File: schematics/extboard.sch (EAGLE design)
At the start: 37 parts, among them X1 FPS009-3000

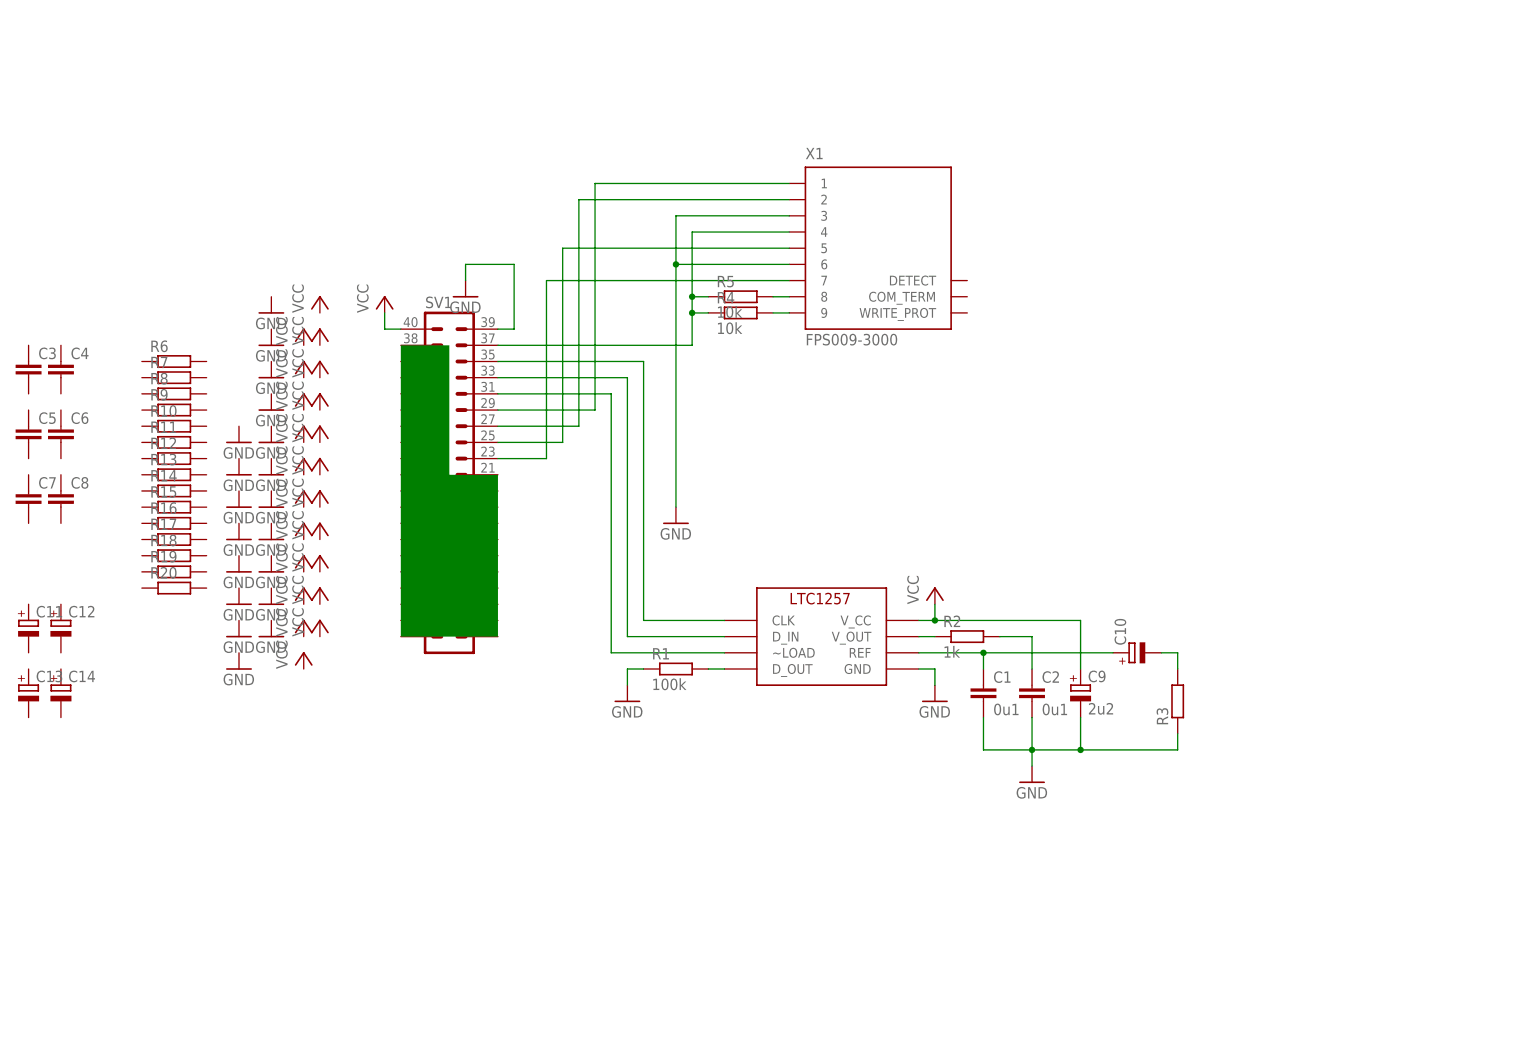
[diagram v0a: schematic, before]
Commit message: schematics: board rev. A
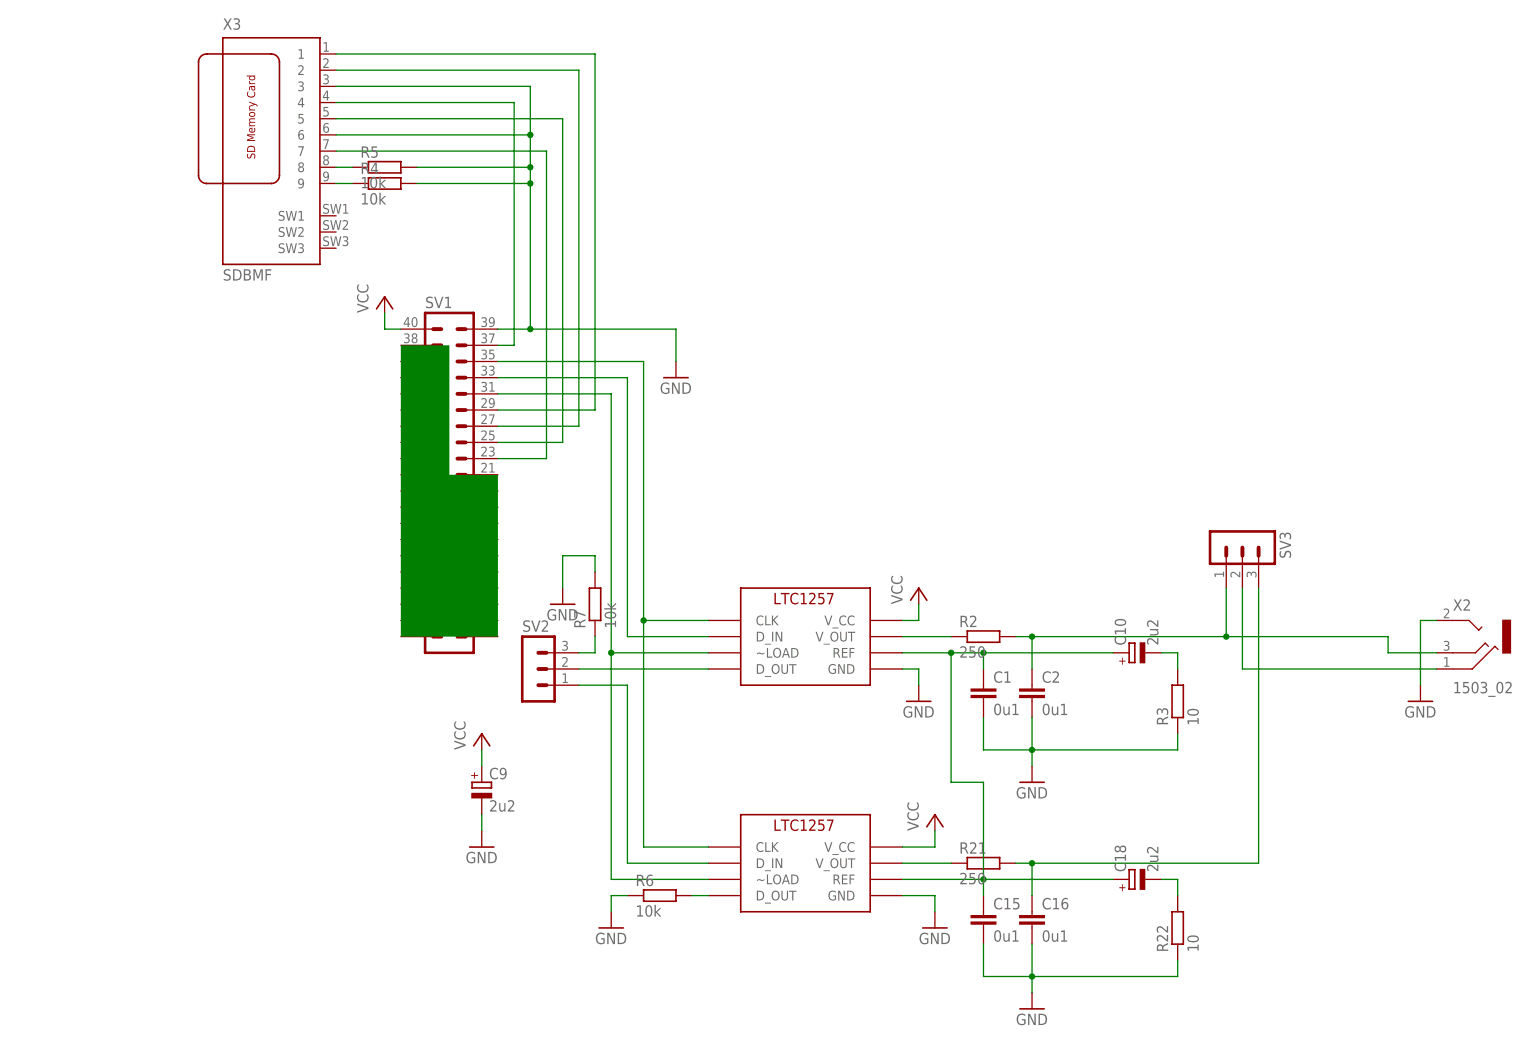
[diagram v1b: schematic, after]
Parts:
- removed C11, C12, C13, C14: (no value), rcl:CPOL-EUE2.5-7
- removed C3, C4, C5, C6, C7, C8: (no value), rcl:C-EU050-035X075
- removed R1: 100k, rcl:R-EU_0207/10
- removed R10, R11, R12, R13, R14, R15, R16, R17, R18, R19, R20, R8, R9: (no value), rcl:R-EU_0207/10
- removed X1: FPS009-3000, con-yamaichi:FPS009-3000
- added C15, C16: 0u1, rcl:C-EU050-035X075
- added C18: 2u2, rcl:CPOL-EUE2.5-7
- added R21: 250, rcl:R-EU_0207/10
- added R22: 10, rcl:R-EU_0207/10
- added SV2, SV3: (no value), con-lstb:MA03-1
- added U$2: LTC1257, ltc1257:LTC1257
- added X2: 1503_02, con-lumberg:1503_02
- added X3: SDBMF, farnell-sd:SDBMF
- C10: value (none) -> 2u2
- R2: value 1k -> 250
- R3: value (none) -> 10
- R6, R7: value (none) -> 10k
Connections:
- new net N$16: R7.1, SV2.3
- new net N$17: SV2.2, U$1.D_OUT
- new net N$18: SV3.2, X2.1
- new net N$19: R6.2, U$2.D_OUT
- new net N$21: C16.1, R21.2, SV3.3
- new net N$22: R21.1, U$2.V_OUT
- new net N$23: C18.-, R22.2
- net GND: now also C15.2, C16.2, R22.1, R4.2, R5.2, R6.1, R7.2, U$2.GND, X2.2, X3.3, X3.6; no longer R1.1, X1.3, X1.6
- net N$1: now also U$2.CLK
- net N$10: now also R4.1, X3.9; no longer R4.2, X1.9
- net N$11: now also X3.4; no longer R4.1, R5.1, X1.4
- net N$12: now also X3.1; no longer X1.1
- net N$13: now also X3.2; no longer X1.2
- net N$14: now also X3.5; no longer X1.5
- net N$15: now also X3.7; no longer X1.7
- net N$3: now also U$2.~LOAD
- net N$4: now also SV2.1, U$2.D_IN; no longer R1.2, U$1.D_OUT
- net N$6: now also C15.1, C18.+, U$2.REF
- net N$7: now also SV3.1, X2.3
- net N$9: now also R5.1, X3.8; no longer R5.2, X1.8
- net VCC: now also U$2.V_CC
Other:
- moved on the sheet: C9, R2, R4, R5, R6, R7
